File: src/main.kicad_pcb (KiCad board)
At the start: 4 copper layers, 24 parts, among them P501 CONN_01X07, Q501 MMBT3904, Q502 MMBT3904, U501 LM741, U502 LM741, U503 2DW232

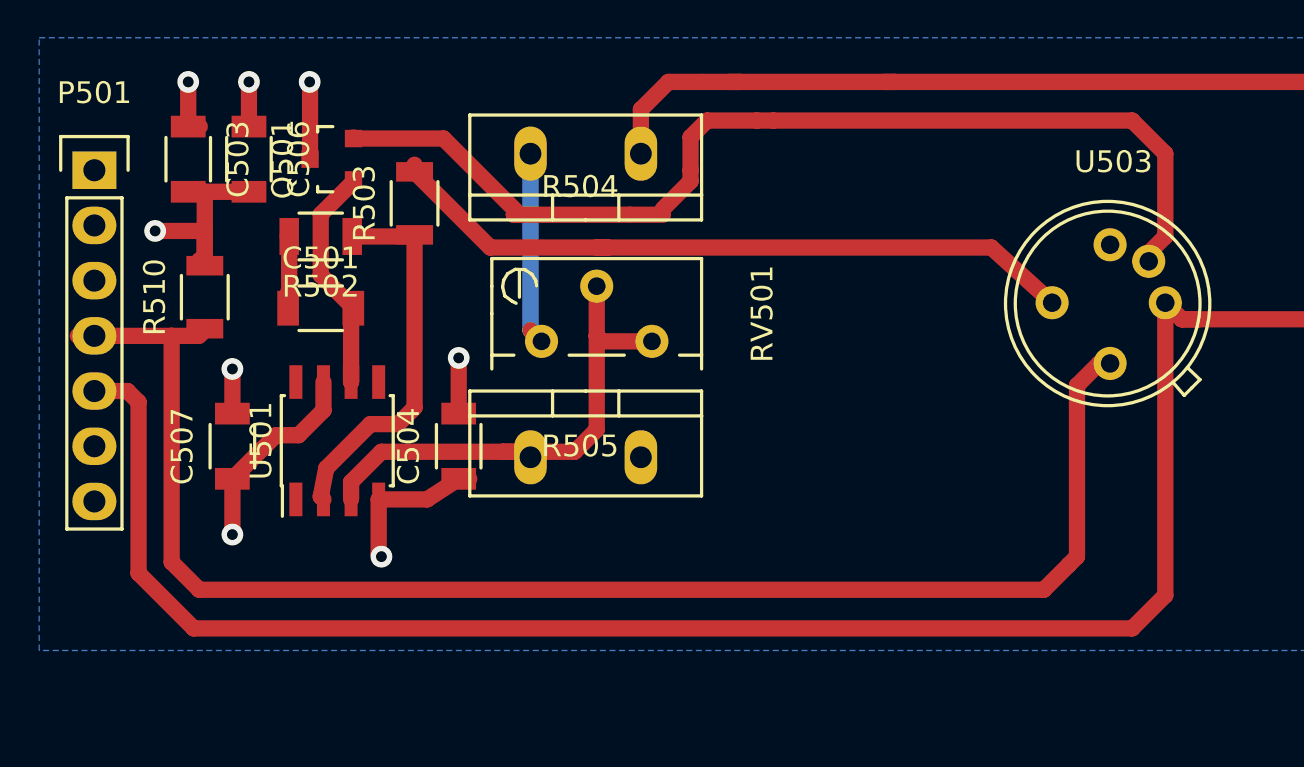
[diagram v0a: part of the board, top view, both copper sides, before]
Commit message: update
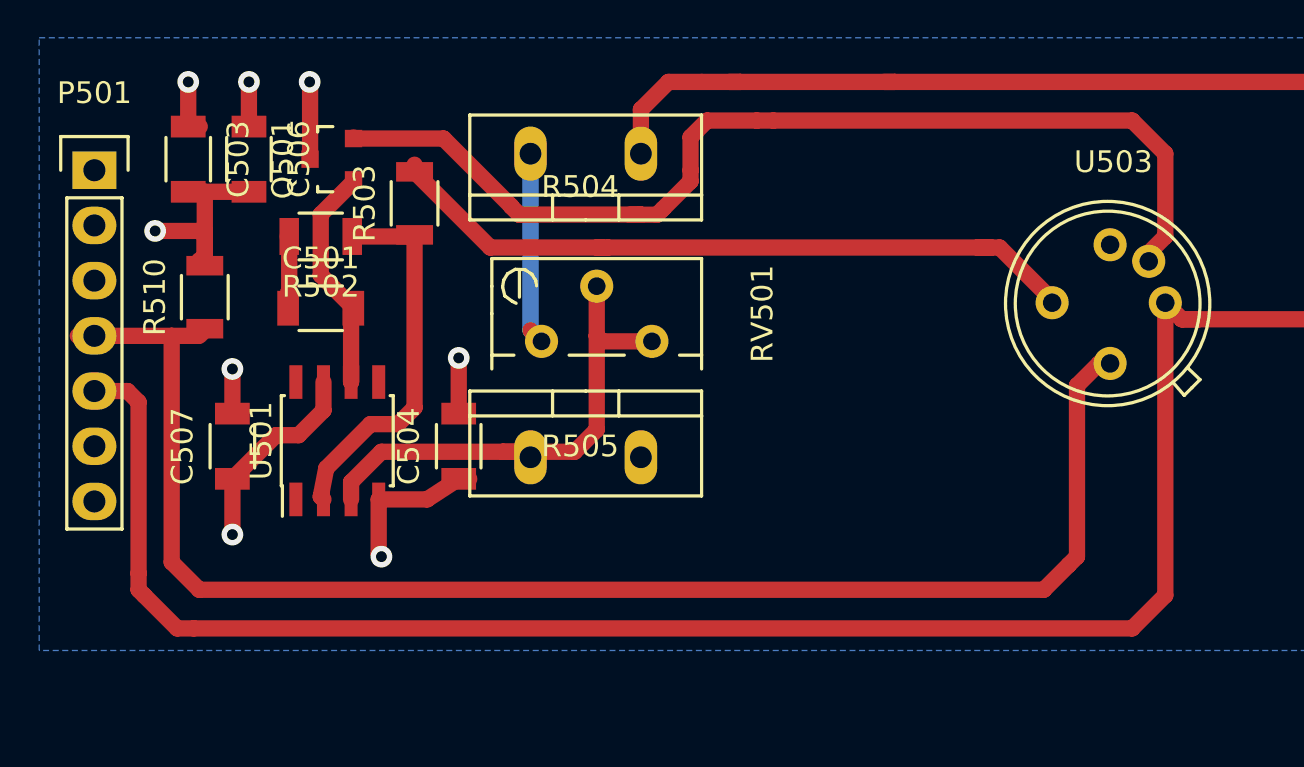
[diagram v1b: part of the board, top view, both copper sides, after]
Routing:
- net Net-(R503-Pad2): track 32.3 -> 33.1 mm
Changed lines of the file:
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@@
     (thickness 1.6)
     (drawings 0)
-    (tracks 212)
+    (tracks 220)
     (zones 0)
     (modules 24)
@@
   (via (at 57.15 53.594) (size 1) (drill 0.5) (layers F.Cu B.Cu) (net 2))
   (segment (start 57.023 53.467) (end 57.15 53.594) (width 0.75) (layer F.Cu) (net 2))
+  (segment (start 48.514 56.896) (end 47.752 56.896) (width 0.75) (layer F.Cu) (net 3))
+  (segment (start 43.942 45.974) (end 45.466 45.974) (width 0.75) (layer F.Cu) (net 3) (status 10))
+  (segment (start 45.974 46.482) (end 45.466 45.974) (width 0.75) (layer F.Cu) (net 3))
+  (segment (start 45.974 54.356) (end 45.974 46.482) (width 0.75) (layer F.Cu) (net 3))
+  (segment (start 93.218 55.372) (end 91.694 56.896) (width 0.75) (layer F.Cu) (net 3))
+  (segment (start 93.218 55.372) (end 93.218 41.91) (width 0.75) (layer F.Cu) (net 3) (status 20))
+  (segment (start 48.514 56.896) (end 91.694 56.896) (width 0.75) (layer F.Cu) (net 3))
+  (segment (start 45.974 55.118) (end 45.974 54.356) (width 0.75) (layer F.Cu) (net 3))
+  (segment (start 46.228 55.372) (end 45.974 55.118) (width 0.75) (layer F.Cu) (net 3))
+  (segment (start 47.752 56.896) (end 46.228 55.372) (width 0.75) (layer F.Cu) (net 3))
   (segment (start 121.158 44.958) (end 119.634 44.958) (width 0.75) (layer F.Cu) (net 3))
   (segment (start 119.634 44.958) (end 117.348 42.672) (width 0.75) (layer F.Cu) (net 3))
@@
   (segment (start 113.284 34.036) (end 111.252 36.068) (width 0.75) (layer F.Cu) (net 3))
   (segment (start 111.252 36.068) (end 111.252 42.672) (width 0.75) (layer F.Cu) (net 3))
-  (segment (start 48.514 56.896) (end 91.694 56.896) (width 0.75) (layer F.Cu) (net 3))
-  (segment (start 93.218 55.372) (end 93.218 41.91) (width 0.75) (layer F.Cu) (net 3) (status 20))
-  (segment (start 93.218 55.372) (end 91.694 56.896) (width 0.75) (layer F.Cu) (net 3))
-  (segment (start 48.514 56.896) (end 45.974 54.356) (width 0.75) (layer F.Cu) (net 3))
-  (segment (start 45.974 54.356) (end 45.974 46.482) (width 0.75) (layer F.Cu) (net 3))
-  (segment (start 45.974 46.482) (end 45.466 45.974) (width 0.75) (layer F.Cu) (net 3))
-  (segment (start 43.942 45.974) (end 45.466 45.974) (width 0.75) (layer F.Cu) (net 3) (status 10))
   (segment (start 93.218 41.91) (end 93.98 42.672) (width 0.75) (layer F.Cu) (net 3) (status 10))
   (segment (start 93.98 42.672) (end 94.742 42.672) (width 0.75) (layer F.Cu) (net 3))
@@
   (segment (start 69.088 35.052) (end 69.088 35.306) (width 0.75) (layer F.Cu) (net 13) (status 30))
   (segment (start 127.74676 35.372) (end 127.74676 35.29076) (width 0.75) (layer F.Cu) (net 13) (status 30))
+  (segment (start 63.492001 37.853999) (end 69.080001 37.853999) (width 0.75) (layer F.Cu) (net 14))
+  (segment (start 69.080001 37.853999) (end 69.088 37.861998) (width 0.75) (layer F.Cu) (net 14))
+  (segment (start 63.119 37.465) (end 63.119 37.480998) (width 0.75) (layer F.Cu) (net 14))
+  (segment (start 63.119 37.480998) (end 63.492001 37.853999) (width 0.75) (layer F.Cu) (net 14))
+  (segment (start 63.492001 37.853999) (end 63.5 37.861998) (width 0.75) (layer F.Cu) (net 14))
+  (segment (start 69.088 37.861998) (end 69.834002 37.861998) (width 0.75) (layer F.Cu) (net 14))
+  (segment (start 69.834002 37.861998) (end 70.104 37.592) (width 0.75) (layer F.Cu) (net 14))
   (segment (start 70.104 37.592) (end 71.374 36.322) (width 0.75) (layer F.Cu) (net 14))
   (segment (start 71.374 36.322) (end 71.374 35.814) (width 0.75) (layer F.Cu) (net 14))
-  (segment (start 63.5 37.861998) (end 63.5 37.846) (width 0.75) (layer F.Cu) (net 14))
-  (segment (start 63.5 37.846) (end 60.01 34.356) (width 0.75) (layer F.Cu) (net 14))
   (segment (start 74.422 33.528) (end 72.136 33.528) (width 0.75) (layer F.Cu) (net 14))
   (segment (start 71.374 34.29) (end 71.374 35.814) (width 0.75) (layer F.Cu) (net 14))
   (segment (start 72.136 33.528) (end 71.374 34.29) (width 0.75) (layer F.Cu) (net 14))
+  (segment (start 75.184 33.528) (end 74.422 33.528) (width 0.75) (layer F.Cu) (net 14))
+  (segment (start 75.184 33.528) (end 91.694 33.528) (width 0.75) (layer F.Cu) (net 14))
+  (segment (start 93.218 38.862) (end 92.456 39.624) (width 0.75) (layer F.Cu) (net 14) (status 20))
+  (segment (start 93.218 35.052) (end 91.694 33.528) (width 0.75) (layer F.Cu) (net 14))
+  (segment (start 93.218 38.862) (end 93.218 35.052) (width 0.75) (layer F.Cu) (net 14))
+  (segment (start 63.119 37.465) (end 60.01 34.356) (width 0.75) (layer F.Cu) (net 14))
   (segment (start 60.01 34.356) (end 55.86476 34.356) (width 0.75) (layer F.Cu) (net 14))
   (segment (start 63.515998 37.861998) (end 63.5 37.861998) (width 0.75) (layer F.Cu) (net 14))
-  (segment (start 63.5 37.861998) (end 63.246 37.861998) (width 0.75) (layer F.Cu) (net 14))
-  (segment (start 63.246 37.846) (end 63.246 37.861998) (width 0.75) (layer F.Cu) (net 14))
-  (segment (start 68.58 37.861998) (end 70.104 37.861998) (width 0.75) (layer F.Cu) (net 14))
-  (segment (start 68.58 37.861998) (end 63.246 37.861998) (width 0.75) (layer F.Cu) (net 14))
-  (segment (start 63.246 37.861998) (end 63.246 37.846) (width 0.75) (layer F.Cu) (net 14))
-  (segment (start 75.184 33.528) (end 74.422 33.528) (width 0.75) (layer F.Cu) (net 14))
-  (segment (start 75.184 33.528) (end 91.694 33.528) (width 0.75) (layer F.Cu) (net 14))
-  (segment (start 92.456 39.624) (end 93.218 38.862) (width 0.75) (layer F.Cu) (net 14) (status 20))
-  (segment (start 93.218 35.052) (end 91.694 33.528) (width 0.75) (layer F.Cu) (net 14))
-  (segment (start 93.218 38.862) (end 93.218 35.052) (width 0.75) (layer F.Cu) (net 14))
+  (segment (start 68.58 37.861998) (end 69.088 37.861998) (width 0.75) (layer F.Cu) (net 14))
   (segment (start 92.456 40.005) (end 92.456 39.624) (width 0.75) (layer F.Cu) (net 14) (status 30))
   (segment (start 92.456 40.005) (end 92.456 39.878) (width 0.75) (layer F.Cu) (net 14) (status 30))
@@
   (segment (start 43.18 43.434) (end 43.942 43.434) (width 0.75) (layer F.Cu) (net 15) (status 30))
   (segment (start 49.022 43.106) (end 48.588 43.106) (width 0.75) (layer F.Cu) (net 15) (status 30))
+  (segment (start 88.011 41.91) (end 88.011 41.783) (width 0.75) (layer F.Cu) (net 16) (status C00000))
+  (segment (start 88.011 41.783) (end 85.598 39.37) (width 0.75) (layer F.Cu) (net 16) (status 400000))
+  (segment (start 85.598 39.37) (end 84.582 39.37) (width 0.75) (layer F.Cu) (net 16))
   (segment (start 67.31 39.37) (end 62.156 39.37) (width 0.75) (layer F.Cu) (net 16))
   (segment (start 62.156 39.37) (end 58.674 35.888) (width 0.75) (layer F.Cu) (net 16))
   (segment (start 67.564 39.37) (end 67.31 39.37) (width 0.75) (layer F.Cu) (net 16))
   (segment (start 67.31 39.37) (end 67.056 39.37) (width 0.75) (layer F.Cu) (net 16))
-  (segment (start 88.011 41.91) (end 85.217 39.37) (width 0.75) (layer F.Cu) (net 16) (status 20))
-  (segment (start 67.564 39.37) (end 85.217 39.37) (width 0.75) (layer F.Cu) (net 16))
+  (segment (start 67.564 39.37) (end 84.582 39.37) (width 0.75) (layer F.Cu) (net 16))
+  (segment (start 84.582 39.37) (end 85.217 39.37) (width 0.75) (layer F.Cu) (net 16))
   (segment (start 58.674 35.56) (end 58.674 35.888) (width 0.75) (layer F.Cu) (net 16) (status 30))
   (zone (net 7) (net_name 0V) (layer In1.Cu) (hatch edge 0.508)
